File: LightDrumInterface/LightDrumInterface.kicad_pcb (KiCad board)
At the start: 2 copper layers, 108 x 83 mm, 74 parts, among them J1 MIDI-IN, J3 DEBUG-CONN, J4 PWR-CONN, J5 MIDI-OUT, J6 0541323662, Q1 NX6008NBKWX, Q2 NX6008NBKWX, Q3 NX6008NBKWX, Q4 NX6008NBKWX, SW1 RESET-SW, U1 STP16CP05, U2 TPL0401B-10-Q1, U3 PC817, U4 74AUP2G04

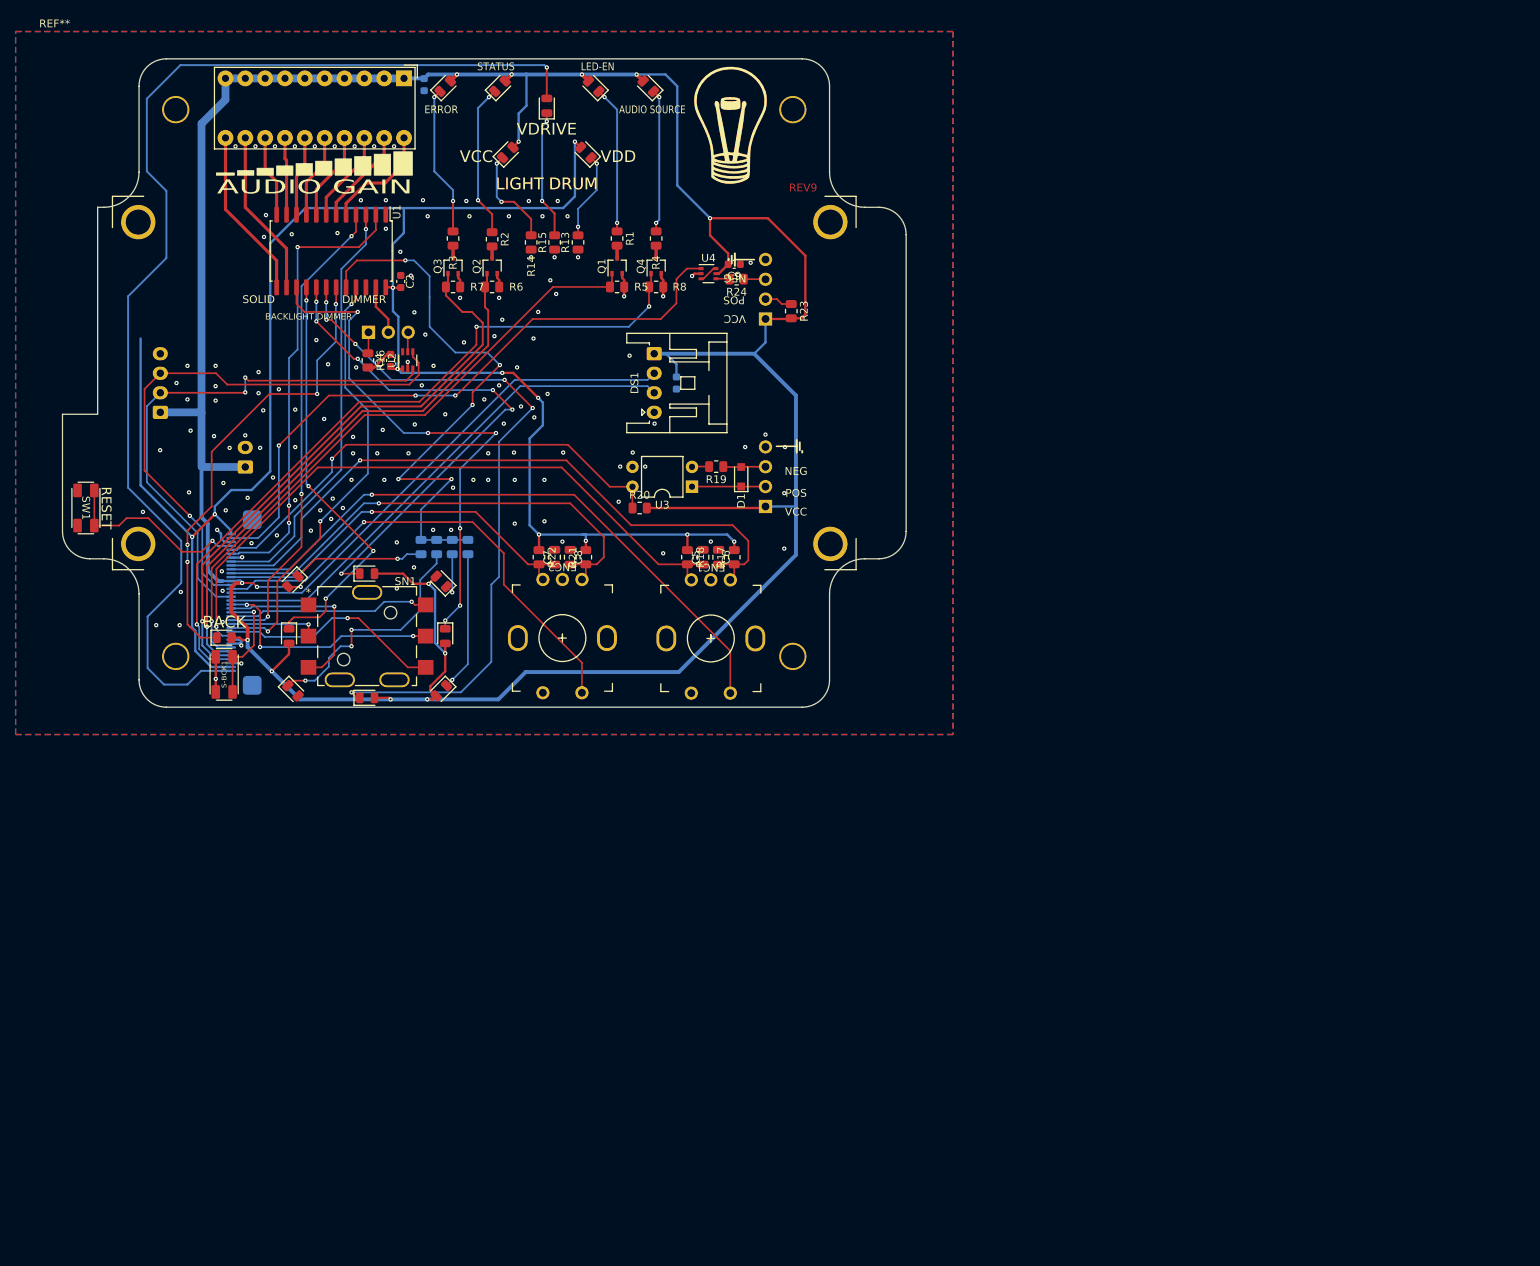
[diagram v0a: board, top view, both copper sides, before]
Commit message: interface layout completed - REV6
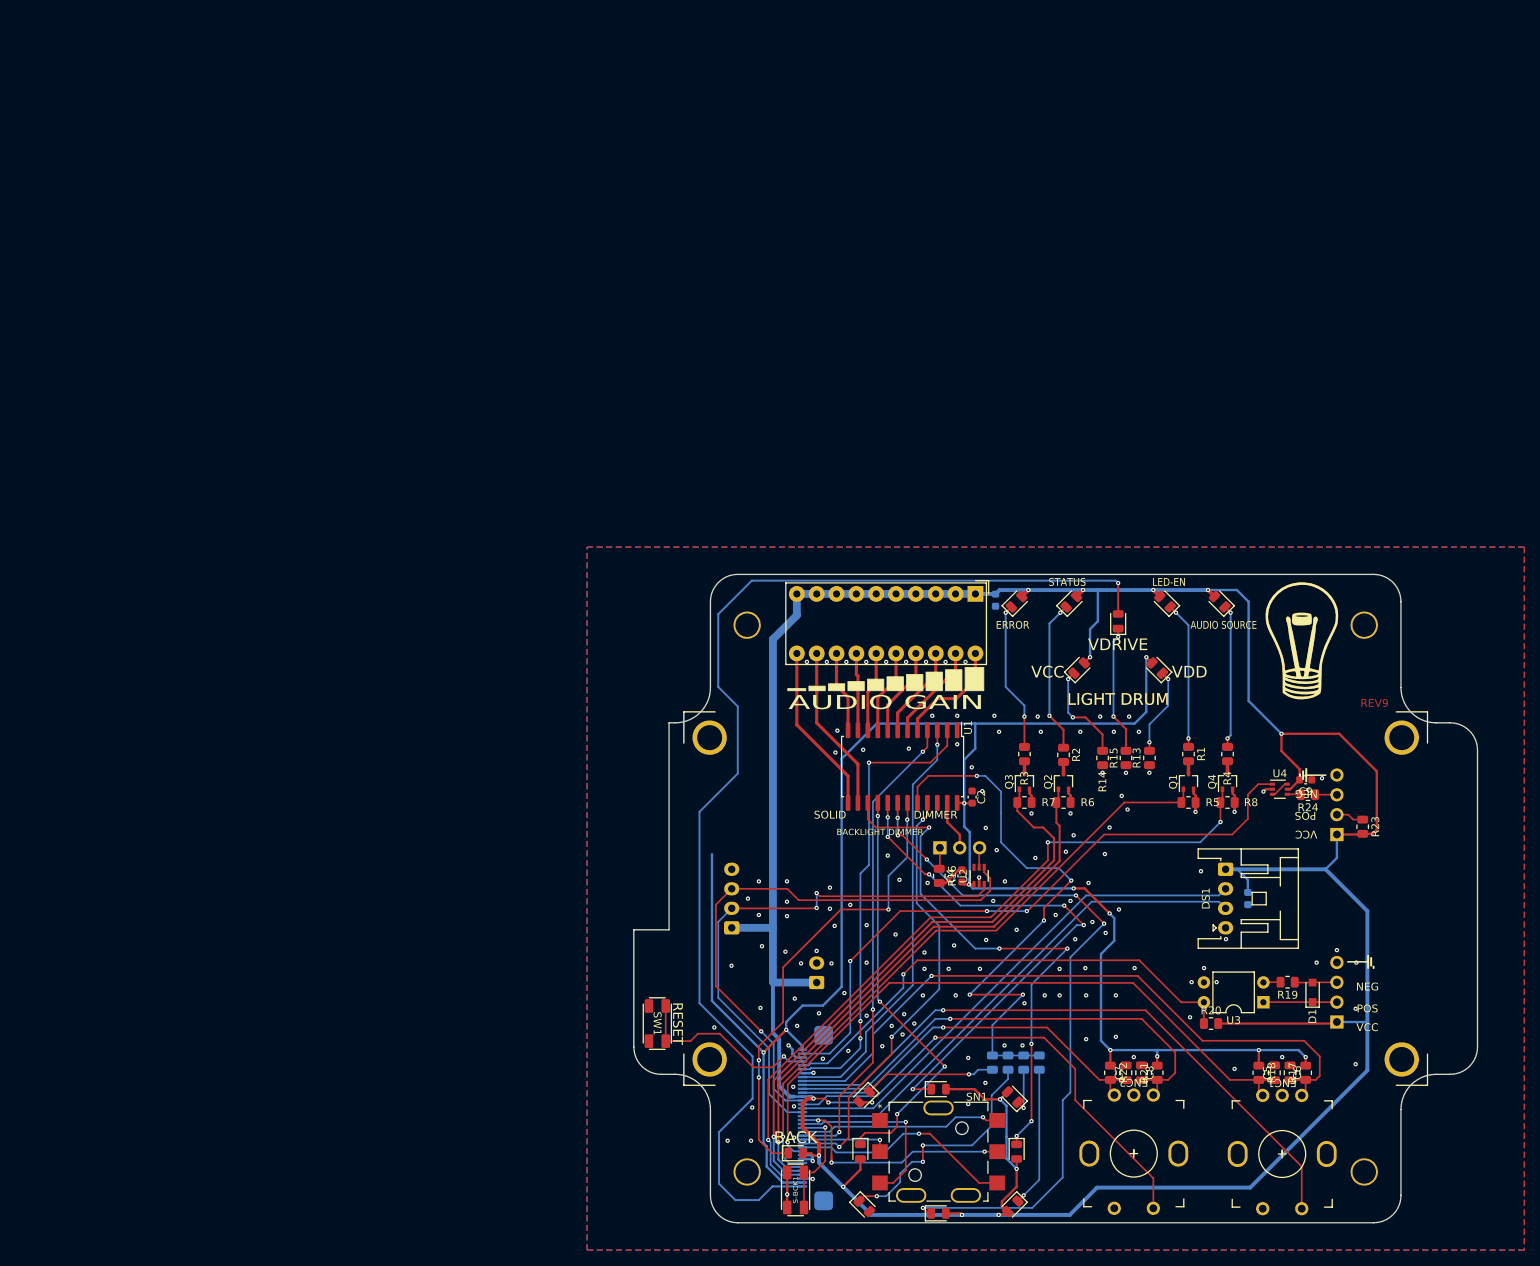
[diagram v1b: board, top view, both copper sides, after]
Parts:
- moved C1 98.5 mm to (97.8, 66.0)
- moved C2 98.5 mm to (62.5, 53.0)
- moved C3 98.5 mm to (65.5, 27.8)
- moved C4 98.5 mm to (61.1, 63.1)
- moved C5 98.5 mm to (103.2, 88.3)
- moved C6 98.5 mm to (101.2, 88.3)
- moved C7 98.5 mm to (84.2, 88.3)
- moved C8 98.5 mm to (82.2, 88.3)
- moved C9 98.5 mm to (105.2, 50.8)
- moved D-AUDIO-SEL1 98.5 mm to (94.2, 28.0)
- moved D-BK1 98.5 mm to (67.7, 91.4)
- moved D-BK2 98.5 mm to (67.7, 105.4)
- moved D-BK3 98.5 mm to (48.6, 105.4)
- moved D-BK4 98.5 mm to (48.6, 91.4)
- moved D-DBG1 98.5 mm to (68.2, 28.0)
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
